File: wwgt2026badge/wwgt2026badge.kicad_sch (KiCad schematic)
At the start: 16 parts, among them J1 Conn_01x08_Pin, J2 Conn_01x04_Pin, SW1 SW_PUSH, SW2 EC12PLGRSDVF, SW3 SW_PUSH, U2 rp2040-zero, U3 fj08k-s

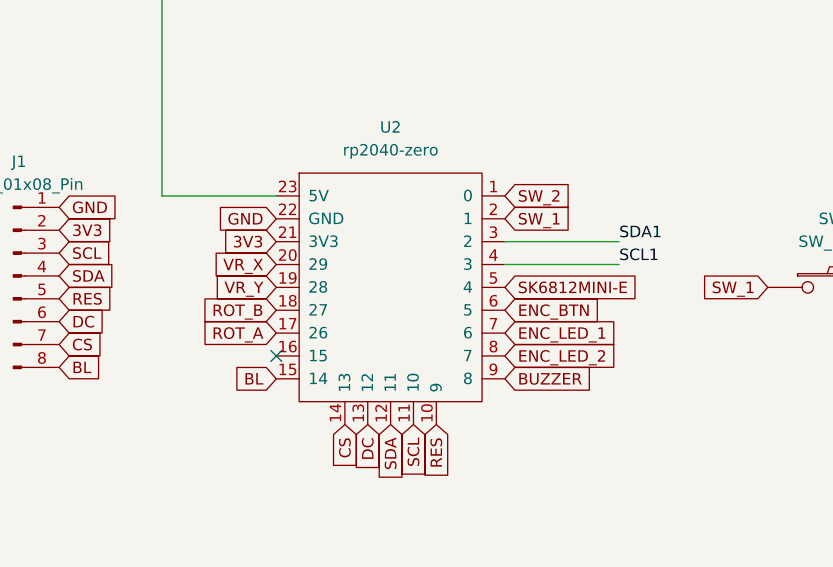
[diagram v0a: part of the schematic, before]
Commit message: updated
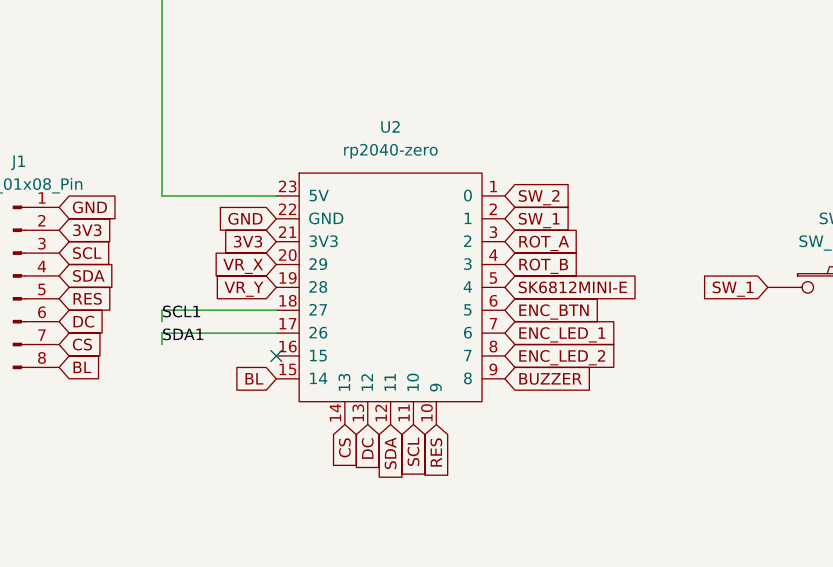
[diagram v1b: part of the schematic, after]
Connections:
- net ROT_A: now also U2.3 (2); no longer U2.17 (26)
- net ROT_B: now also U2.4 (3); no longer U2.18 (27)
- net SCL1: now also U2.18 (27); no longer U2.4 (3)
- net SDA1: now also U2.17 (26); no longer U2.3 (2)
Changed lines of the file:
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@@
+	(wire
+		(pts
+			(xy 52.07 91.44) (xy 39.37 91.44)
+		)
+		(stroke
+			(width 0)
+			(type default)
+		)
+	)
 	(wire
 		(pts
@@
 	(wire
 		(pts
-			(xy 77.47 83.82) (xy 90.17 83.82)
-		)
-		(stroke
-			(width 0)
-			(type default)
-		)
-	)
-	(wire
-		(pts
 			(xy 73.66 149.86) (xy 88.9 149.86)
 		)
@@
 	(wire
 		(pts
-			(xy 77.47 86.36) (xy 90.17 86.36)
-		)
-		(stroke
-			(width 0)
-			(type default)
-		)
-	)
-	(wire
-		(pts
 			(xy 142.24 48.26) (xy 121.92 48.26)
 		)
@@
 	(wire
 		(pts
+			(xy 52.07 93.98) (xy 39.37 93.98)
+		)
+		(stroke
+			(width 0)
+			(type default)
+		)
+	)
+	(wire
+		(pts
 			(xy 177.8 90.17) (xy 190.5 90.17)
 		)
@@
 	(wire
 		(pts
+			(xy 39.37 91.44) (xy 39.37 92.71)
+		)
+		(stroke
+			(width 0)
+			(type default)
+		)
+	)
+	(wire
+		(pts
 			(xy 177.8 92.71) (xy 200.66 92.71)
 		)
@@
 	(wire
 		(pts
+			(xy 39.37 93.98) (xy 39.37 95.25)
+		)
+		(stroke
+			(width 0)
+			(type default)
+		)
+	)
+	(wire
+		(pts
 			(xy 83.82 144.78) (xy 83.82 160.02)
 		)
@@
 	)
 	(label "SDA1"
-		(at 90.17 83.82 0)
+		(at 39.37 95.25 0)
 		(effects
 			(font
@@
 	)
 	(label "SCL1"
-		(at 90.17 86.36 0)
+		(at 39.37 92.71 0)
 		(effects
 			(font
@@
 	(global_label "ROT_A"
 		(shape input)
-		(at 52.07 93.98 180)
-		(fields_autoplaced yes)
-		(effects
-			(font
-				(size 1.27 1.27)
-			)
-			(justify right)
-		)
-		(property "Intersheetrefs" "${INTERSHEET_REFS}"
-			(at 43.4605 93.98 0)
-			(effects
-				(font
-					(size 1.27 1.27)
-				)
-				(justify right)
+		(at 77.47 83.82 0)
+		(fields_autoplaced yes)
+		(effects
+			(font
+				(size 1.27 1.27)
+			)
+			(justify left)
+		)
+		(property "Intersheetrefs" "${INTERSHEET_REFS}"
+			(at 86.0795 83.82 0)
+			(effects
+				(font
+					(size 1.27 1.27)
+				)
+				(justify left)
 				(hide yes)
 			)
@@
 	(global_label "ROT_B"
 		(shape input)
-		(at 52.07 91.44 180)
-		(fields_autoplaced yes)
-		(effects
-			(font
-				(size 1.27 1.27)
-			)
-			(justify right)
-		)
-		(property "Intersheetrefs" "${INTERSHEET_REFS}"
-			(at 43.2791 91.44 0)
-			(effects
-				(font
-					(size 1.27 1.27)
-				)
-				(justify right)
-				(hide yes)
-			)
+		(at 77.47 86.36 0)
+		(fields_autoplaced yes)
+		(effects
+			(font
+				(size 1.27 1.27)
+			)
+			(justify left)
+		)
+		(property "Intersheetrefs" "${INTERSHEET_REFS}"
+			(at 86.2609 86.36 0)
+			(effects
+				(font
+					(size 1.27 1.27)
+				)
+				(justify left)
+				(hide yes)
+			)
